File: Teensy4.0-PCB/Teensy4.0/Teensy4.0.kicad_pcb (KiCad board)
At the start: 4 copper layers, 76 x 58 mm, 74 parts, among them IC2 NC7WZ241K8X, J1 24-27, J2 28-31, U1 Teensy4.0, U2 NRF24, U3 TXS0104ERGYR, U4 TPS62143RGTT, U5 MIC5504-1.8YM5, U6 ICM-20948, U7 TXS0104ERGYR, U8 MMBT8099LT1G

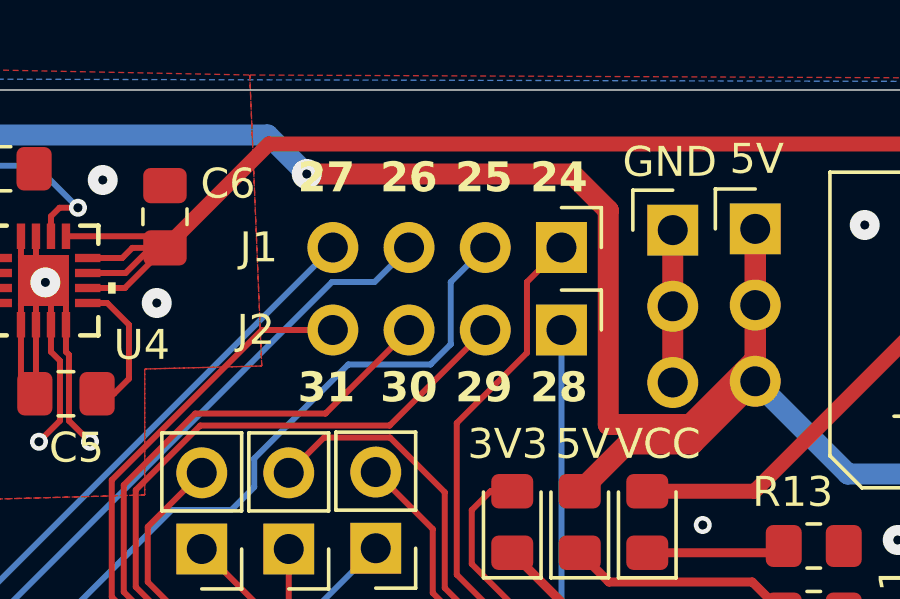
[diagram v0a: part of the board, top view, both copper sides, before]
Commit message: changed some stuff
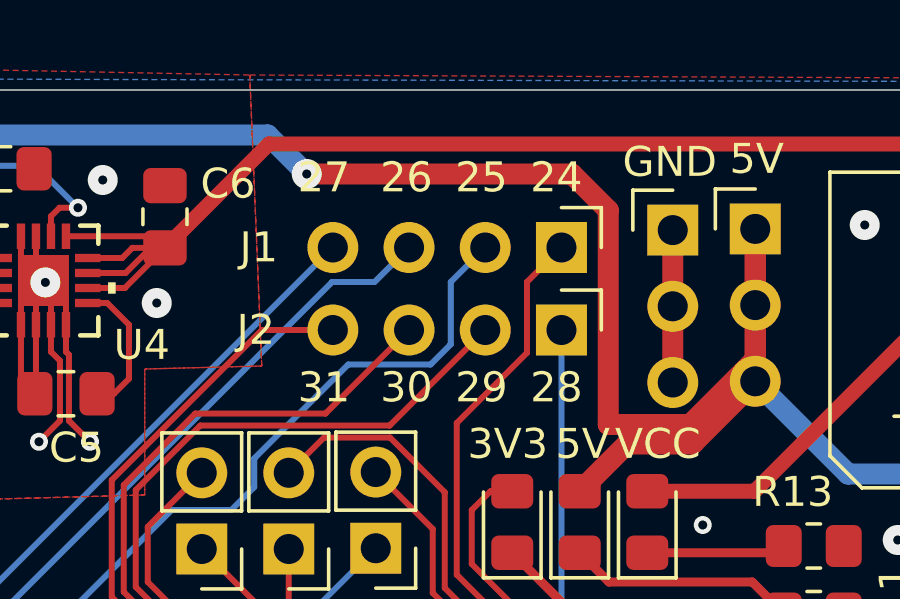
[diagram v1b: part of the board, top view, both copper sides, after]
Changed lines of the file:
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@@
 			(pintype "passive")
 		)
-		(model "/home/jirakornsukmee/Documents/Morphing-Robot/Teensy4.0-PCB/models/IND_SRP2512_BRN.step"
+		(model "/Users/jirakornsukmee/Documents/Morphing-Robot/Teensy4.0-PCB/models/IND_SRP2512_BRN.step"
 			(offset
 				(xyz 0 0 0)
@@
 			(font
 				(size 1 1)
-				(thickness 0.25)
-				(bold yes)
+				(thickness 0.15)
 			)
 			(justify left bottom)
@@
 			(font
 				(size 1 1)
-				(thickness 0.25)
-				(bold yes)
+				(thickness 0.15)
 			)
 			(justify left bottom)
@@
 			(font
 				(size 1 1)
-				(thickness 0.25)
-				(bold yes)
+				(thickness 0.15)
 			)
 			(justify left bottom)
@@
 			(font
 				(size 1 1)
-				(thickness 0.25)
-				(bold yes)
+				(thickness 0.15)
 			)
 			(justify left bottom)
@@
 			(font
 				(size 1 1)
-				(thickness 0.25)
-				(bold yes)
+				(thickness 0.15)
 			)
 			(justify left bottom)
@@
 			(font
 				(size 1 1)
-				(thickness 0.25)
-				(bold yes)
+				(thickness 0.15)
 			)
 			(justify left bottom)
@@
 			(font
 				(size 1 1)
-				(thickness 0.25)
-				(bold yes)
+				(thickness 0.15)
 			)
 			(justify left bottom)
@@
 			(font
 				(size 1 1)
-				(thickness 0.25)
-				(bold yes)
+				(thickness 0.15)
 			)
 			(justify left bottom)
@@
 	)
 	(zone
-		(net 0)
-		(net_name "")
-		(layer "F.Cu")
-		(hatch edge 0.5)
-		(connect_pads
-			(clearance 0)
-		)
-		(min_thickness 0.25)
-		(filled_areas_thickness no)
-		(keepout
-			(tracks allowed)
-			(vias allowed)
-			(pads allowed)
-			(copperpour not_allowed)
-			(footprints allowed)
-		)
-		(fill
-			(thermal_gap 0.5)
-			(thermal_bridge_width 0.5)
-		)
-		(polygon
-			(pts
-				(xy 149.748 104.7) (xy 149.748 102.1) (xy 152.548 102.1) (xy 152.548 104.7)
-			)
-		)
-	)
-	(zone
 		(net 5)
 		(net_name "GND")
@@
 			)
 		)
+	)
+	(zone
+		(net 0)
+		(net_name "")
+		(layers "F.Cu" "In1.Cu" "In2.Cu" "B.Cu")
+		(hatch edge 0.5)
+		(connect_pads
+			(clearance 0)
+		)
+		(min_thickness 0.25)
+		(filled_areas_thickness no)
+		(keepout
+			(tracks allowed)
+			(vias allowed)
+			(pads allowed)
+			(copperpour not_allowed)
+			(footprints allowed)
+		)
+		(fill
+			(thermal_gap 0.5)
+			(thermal_bridge_width 0.5)
+		)
+		(polygon
+			(pts
+				(xy 149.748 104.7) (xy 149.748 102.1) (xy 152.548 102.1) (xy 152.548 104.7)
+			)
+		)
